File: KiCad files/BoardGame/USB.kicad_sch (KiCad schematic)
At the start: 12 parts, among them J201 USB_C_Receptacle_USB2.0, U201 USBLC6-2SC6, U202 CH340C

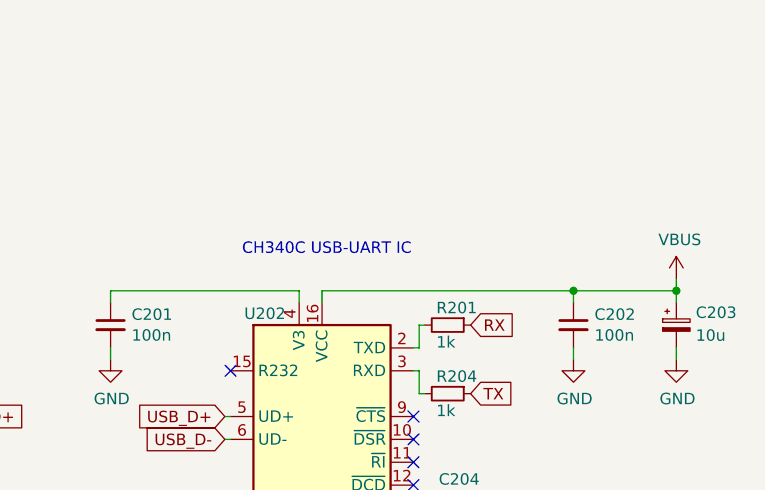
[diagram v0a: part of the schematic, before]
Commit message: update
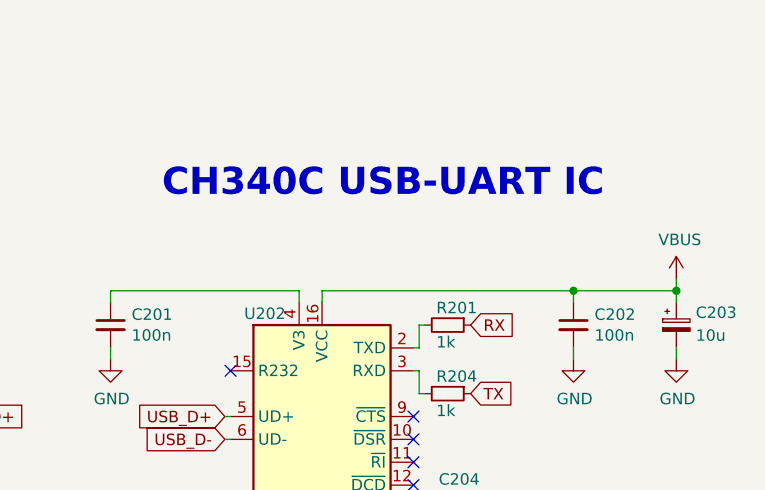
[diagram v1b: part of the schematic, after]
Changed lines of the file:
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@@
     (effects (font (size 1.27 1.27)) (justify left bottom))
   )
-  (text "CH340C USB-UART IC" (at 219.075 71.12 0)
-    (effects (font (size 1.27 1.27)) (justify left bottom))
+  (text "CH340C USB-UART IC" (at 210.185 64.77 0)
+    (effects (font (size 3 3) (thickness 0.6) bold) (justify left bottom))
   )
   (text "ESD protection IC" (at 161.29 105.41 0)
